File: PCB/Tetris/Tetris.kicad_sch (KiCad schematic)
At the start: 41 parts, among them J2 PWM, J3 Analog, J4 PWM, J5 Analog, J6 Communication, J7 Digital, M1 RGBMatrix, M2 RGBMatrix, SW1 SW_Push, SW2 SW_Push, SW3 SW_Push, SW4 SW_Push, SW5 SW_Push, SW6 SW_Push, SW7 SW_Push

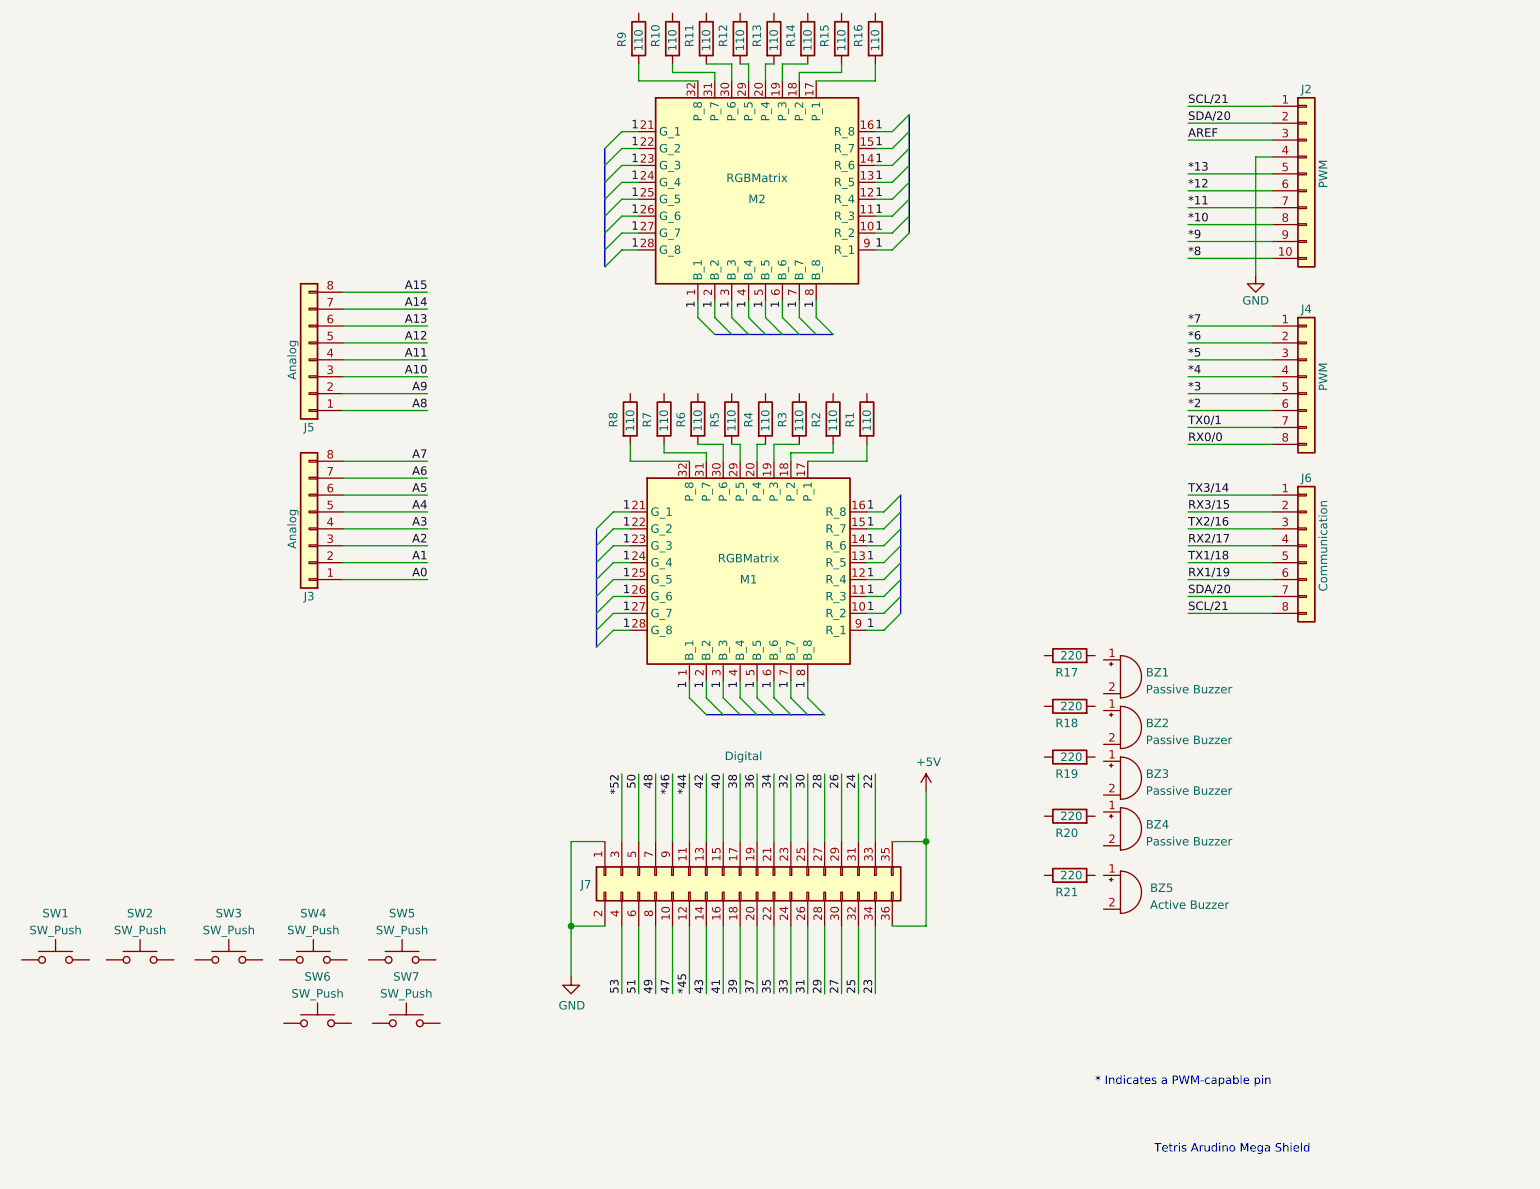
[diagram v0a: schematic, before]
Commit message: sync
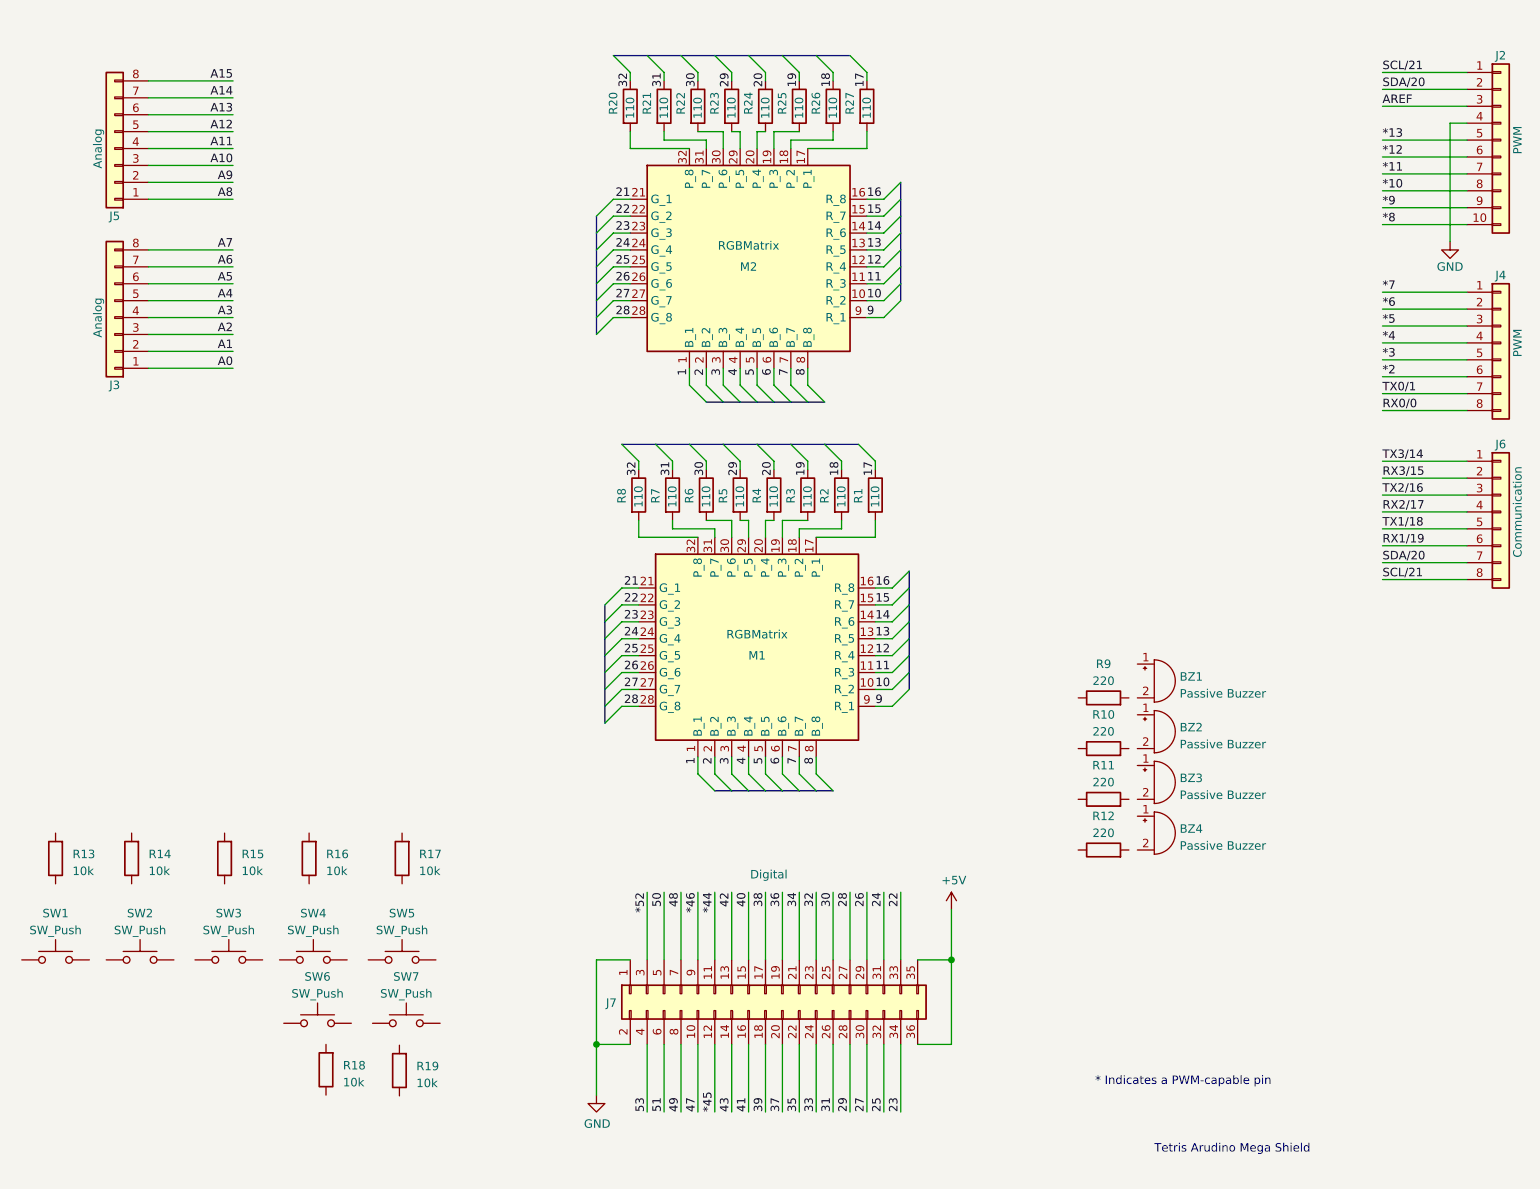
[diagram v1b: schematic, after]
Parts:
- removed BZ5: Active Buzzer, Buzzer_Beeper:MagneticBuzzer_PUI_AT-0927-TT-6-R, symbol Device:Buzzer
- added R22, R23, R24, R25, R26, R27: 110, Resistor_THT:R_Axial_DIN0207_L6.3mm_D2.5mm_P10.16mm_Horizontal, symbol Device:R
- BZ1, BZ2, BZ3, BZ4: footprint Buzzer_Beeper:MagneticBuzzer_PUI_AT-0927-TT-6-R -> Buzzer_Beeper:Buzzer_TDK_PS1240P02BT_D12.2mm_H6.5mm
- J2: footprint Connector_PinSocket_2.54mm:PinSocket_1x10_P2.54mm_Vertical -> Connector_PinHeader_2.54mm:PinHeader_1x10_P2.54mm_Vertical
- J4, J6: footprint Connector_PinSocket_2.54mm:PinSocket_1x08_P2.54mm_Vertical -> Connector_PinHeader_2.54mm:PinHeader_1x08_P2.54mm_Vertical
- R1, R2, R3, R4, R5, R6, R7, R8: footprint (none) -> Resistor_THT:R_Axial_DIN0207_L6.3mm_D2.5mm_P10.16mm_Horizontal
- R10, R11, R12, R9: value 110 -> 220; footprint (none) -> Resistor_THT:R_Axial_DIN0207_L6.3mm_D2.5mm_P10.16mm_Horizontal
- R13, R14, R15, R16: value 110 -> 10k; footprint (none) -> Resistor_THT:R_Axial_DIN0207_L6.3mm_D2.5mm_P10.16mm_Horizontal
- R17, R18, R19: value 220 -> 10k; footprint (none) -> Resistor_THT:R_Axial_DIN0207_L6.3mm_D2.5mm_P10.16mm_Horizontal
- R20, R21: value 220 -> 110; footprint (none) -> Resistor_THT:R_Axial_DIN0207_L6.3mm_D2.5mm_P10.16mm_Horizontal
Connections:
- net 1: no longer M1.10 (R_2), M1.11 (R_3), M1.12 (R_4), M1.13 (R_5), M1.14 (R_6), M1.15 (R_7), M1.16 (R_8), M1.2 (B_2), M1.21 (G_1), M1.22 (G_2), M1.23 (G_3), M1.24 (G_4), M1.25 (G_5), M1.26 (G_6), M1.27 (G_7), M1.28 (G_8), M1.3 (B_3), M1.4 (B_4), M1.5 (B_5), M1.6 (B_6), M1.7 (B_7), M1.8 (B_8), M1.9 (R_1), M2.10 (R_2), M2.11 (R_3), M2.12 (R_4), M2.13 (R_5), M2.14 (R_6), M2.15 (R_7), M2.16 (R_8), M2.2 (B_2), M2.21 (G_1), M2.22 (G_2), M2.23 (G_3), M2.24 (G_4), M2.25 (G_5), M2.26 (G_6), M2.27 (G_7), M2.28 (G_8), M2.3 (B_3), M2.4 (B_4), M2.5 (B_5), M2.6 (B_6), M2.7 (B_7), M2.8 (B_8), M2.9 (R_1)
- net 22: now also M1.22 (G_2), M2.22 (G_2)
- net 23: now also M1.23 (G_3), M2.23 (G_3)
- net 24: now also M1.24 (G_4), M2.24 (G_4)
- net 25: now also M1.25 (G_5), M2.25 (G_5)
- net 26: now also M1.26 (G_6), M2.26 (G_6)
- net 27: now also M1.27 (G_7), M2.27 (G_7)
- net 28: now also M1.28 (G_8), M2.28 (G_8)
- net 29: now also R5.1, R23.1
- net 30: now also R6.1, R22.1
- net 31: now also R21.1, R7.1
- net 32: now also R20.1, R8.1
- net at R16.2: no longer M2.17 (P_1)
- net at R10.2: no longer M2.31 (P_7)
- net at M2.29 (P_5): now also R23.2; no longer R12.2
- net at M2.18 (P_2): now also R26.2; no longer R15.2
- net at M2.19 (P_3): now also R25.2; no longer R14.2
- net at M2.20 (P_4): now also R24.2; no longer R13.2
- net at M2.30 (P_6): now also R22.2; no longer R11.2
- net at M2.32 (P_8): now also R20.2; no longer R9.2
- net 20: now reaches R4.1
- net 20: now also R24.1
- net 19: now reaches R3.1
- net 19: now also R25.1
- net 18: now reaches R2.1
- net 18: now also R26.1
- net 17: now reaches R1.1
- net 17: now also R27.1
- net at R21.2: now also M2.31 (P_7)
- new net: M2.17 (P_1), R27.2
- new net 10: M1.10 (R_2), M2.10 (R_2)
- new net 11: M1.11 (R_3), M2.11 (R_3)
- new net 12: M1.12 (R_4), M2.12 (R_4)
- new net 13: M1.13 (R_5), M2.13 (R_5)
- new net 14: M1.14 (R_6), M2.14 (R_6)
- new net 15: M1.15 (R_7), M2.15 (R_7)
- new net 16: M1.16 (R_8), M2.16 (R_8)
- new net 2: M1.2 (B_2), M2.2 (B_2)
- new net 21: M1.21 (G_1), M2.21 (G_1)
- new net 3: M1.3 (B_3), M2.3 (B_3)
- new net 4: M1.4 (B_4), M2.4 (B_4)
- new net 5: M1.5 (B_5), M2.5 (B_5)
- new net 6: M1.6 (B_6), M2.6 (B_6)
- new net 7: M1.7 (B_7), M2.7 (B_7)
- new net 8: M1.8 (B_8), M2.8 (B_8)
- new net 9: M1.9 (R_1), M2.9 (R_1)
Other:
- moved on the sheet: BZ1, BZ2, BZ3, BZ4, J2, J3, J4, J5, J6, J7, M1, R1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

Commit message: Making diabolical progress
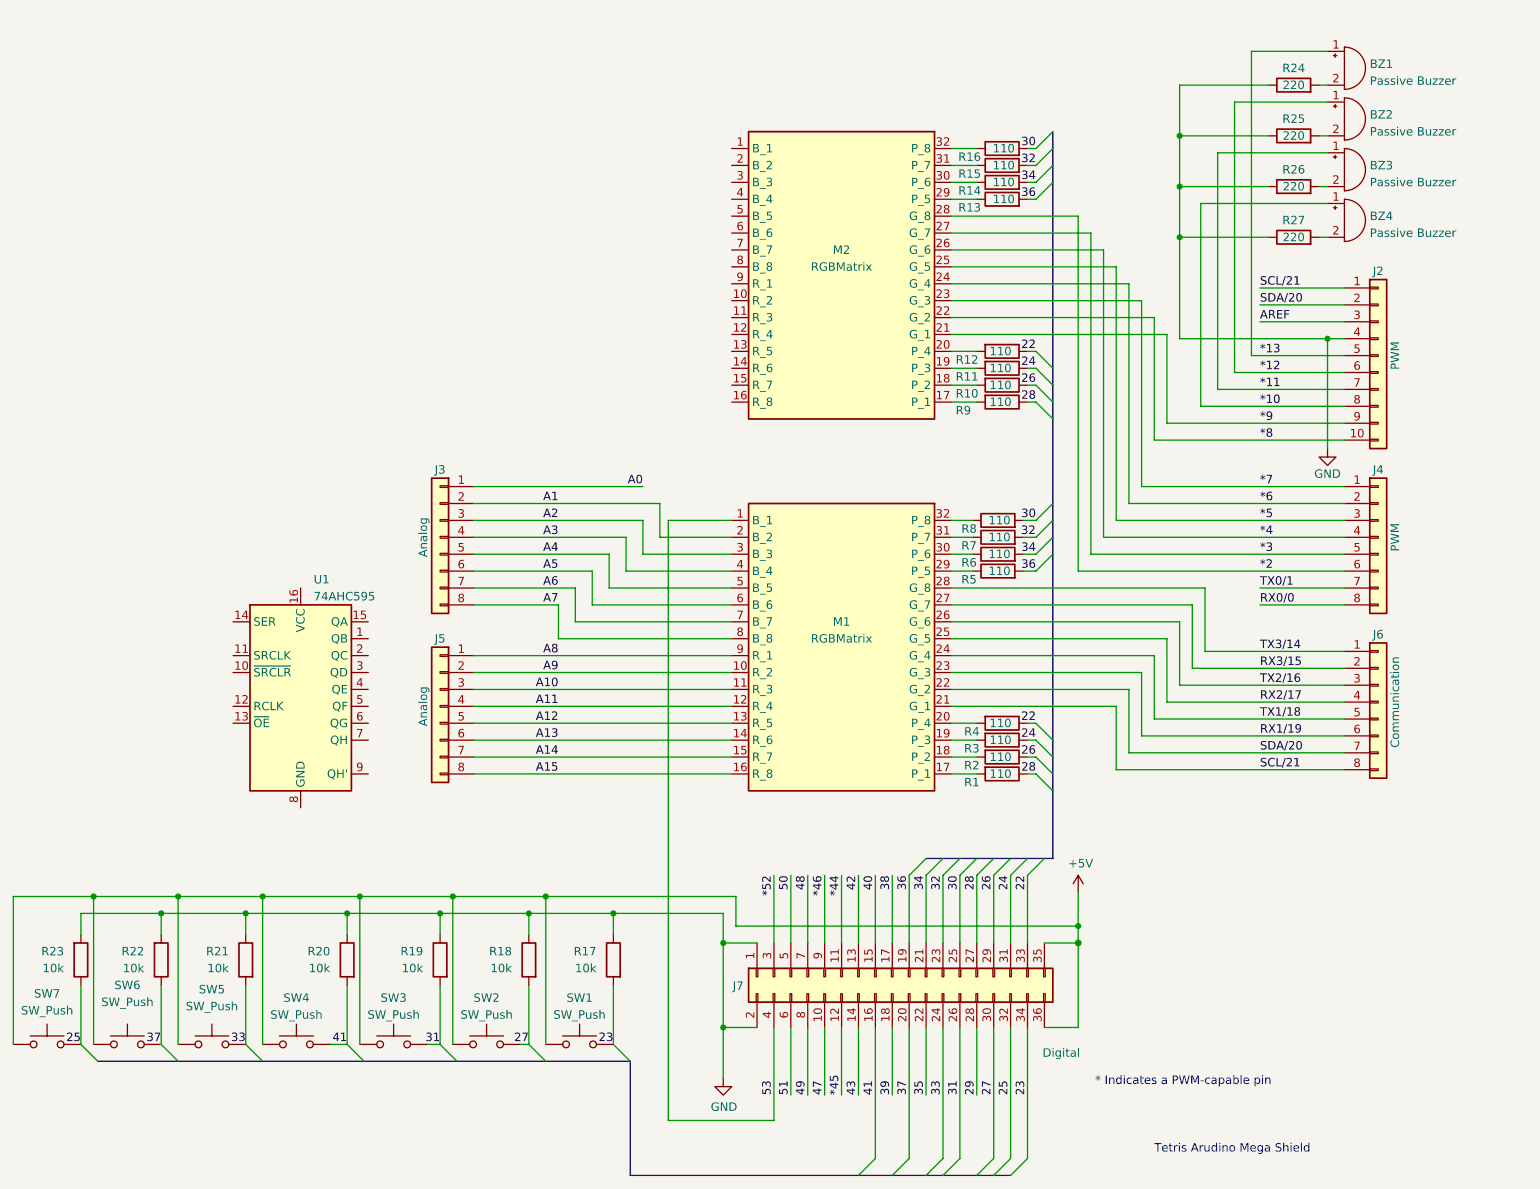
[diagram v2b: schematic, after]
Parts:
- removed R20, R21, R22, R23, R24, R25, R26, R27: 110, Resistor_THT:R_Axial_DIN0207_L6.3mm_D2.5mm_P10.16mm_Horizontal, symbol Device:R
- added R10, R11, R12, R13, R14, R15, R16, R9: 110, Resistor_THT:R_Axial_DIN0207_L6.3mm_D2.5mm_P10.16mm_Horizontal, symbol Device:R
- added U1: 74AHC595, Package_DIP:DIP-16_W7.62mm_Socket_LongPads, symbol 74xx:74AHC595
- J3, J5: footprint Connector_PinSocket_2.54mm:PinSocket_1x08_P2.54mm_Vertical -> Connector_PinHeader_2.54mm:PinHeader_1x08_P2.54mm_Vertical
- J7: footprint Connector_PinSocket_2.54mm:PinSocket_2x18_P2.54mm_Vertical -> Connector_PinHeader_2.54mm:PinHeader_2x18_P2.54mm_Vertical
- renumbered R13 to R17, R14 to R18, R15 to R19, R16 to R20, R17 to R21, R18 to R22, R19 to R23, R9 to R24, R10 to R25, R11 to R26, R12 to R27, R8 to R5, R7 to R6, R6 to R7, R5 to R8
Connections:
- net 17 is gone; now on net 28: R1.1
- net 18 is gone; now on net 26: R2.1
- net 19 is gone; now on net 24: R3.1
- net 20 is gone; now on net 22: R4.1
- net *10: now also BZ4.1 (-)
- net *11: now also BZ3.1 (-)
- net *12: now also BZ2.1 (-)
- net *13: now also BZ1.1 (-)
- net *2: now also M2.28 (G_8)
- net *3: now also M2.27 (G_7)
- net *4: now also M2.26 (G_6)
- net *5: now also M2.25 (G_5)
- net *6: now also M2.24 (G_4)
- net *7: now also M2.23 (G_3)
- net *8: now also M2.22 (G_2)
- net *9: now also M2.21 (G_1)
- net +5V: now also SW1.2, SW2.2, SW3.2, SW4.2, SW5.2, SW6.2, SW7.2
- net 22: now also R12.1; no longer M1.22 (G_2), M2.22 (G_2)
- net 23: now also R17.2, SW1.1; no longer M1.23 (G_3), M2.23 (G_3)
- net 24: now also R11.1; no longer M1.24 (G_4), M2.24 (G_4)
- net 25: now also R23.1, SW7.1; no longer M1.25 (G_5), M2.25 (G_5)
- net 26: now also R10.1; no longer M1.26 (G_6), M2.26 (G_6)
- net 27: now also R18.2, SW2.1; no longer M1.27 (G_7), M2.27 (G_7)
- net 28: now also R9.1; no longer M1.28 (G_8), M2.28 (G_8)
- net 29: no longer R8.1
- net 30: now also R8.2, R16.2; no longer R7.1
- net 31: now also R19.2, SW3.1; no longer R6.1
- net 32: now also R7.2, R15.2; no longer R5.1
- net 33: now also R21.2, SW5.1
- net 34: now also R6.2, R14.2
- net 36: now also R5.2, R13.2
- net 37: now also R22.1, SW6.1
- net 41: now also R20.2, SW4.1
- net 53: now also M1.1 (B_1)
- net A1: now also M1.2 (B_2)
- net A10: now also M1.11 (R_3)
- net A11: now also M1.12 (R_4)
- net A12: now also M1.13 (R_5)
- net A13: now also M1.14 (R_6)
- net A14: now also M1.15 (R_7)
- net A15: now also M1.16 (R_8)
- net A2: now also M1.3 (B_3)
- net A3: now also M1.4 (B_4)
- net A4: now also M1.5 (B_5)
- net A5: now also M1.6 (B_6)
- net A6: now also M1.7 (B_7)
- net A7: now also M1.8 (B_8)
- net A8: now also M1.9 (R_1)
- net A9: now also M1.10 (R_2)
- net GND: now also R17.1, R18.1, R19.1, R20.1, R21.1, R22.2, R23.2, R24.1, R25.1, R26.1, R27.1
- net RX1/19: now also M1.23 (G_3)
- net RX2/17: now also M1.25 (G_5)
- net RX3/15: now also M1.27 (G_7)
- net SCL/21: now also M1.21 (G_1)
- net SDA/20: now also M1.22 (G_2)
- net TX1/18: now also M1.24 (G_4)
- net TX2/16: now also M1.26 (G_6)
- net TX3/14: now also M1.28 (G_8)
- net at BZ1.2 (+): now also R24.2
- net at M2.20 (P_4): now also R12.2
- net at R25.2: now also BZ2.2 (+)
- net at BZ3.2 (+): now also R26.2
- net at M2.17 (P_1): now also R9.2
- net at M2.18 (P_2): now also R10.2
- net at M2.19 (P_3): now also R11.2
- net at M2.29 (P_5): now also R13.1
- net at M2.30 (P_6): now also R14.1
- net at M2.31 (P_7): now also R15.1
- net at M2.32 (P_8): now also R16.1
- net at M1.32 (P_8): now also R8.1; no longer R5.2
- net at M1.31 (P_7): now also R7.1; no longer R6.2
- net at M1.30 (P_6): now also R6.1; no longer R7.2
- net at BZ4.2 (+): now also R27.2
- net at M1.29 (P_5): now also R5.1; no longer R8.2
- net 1: no longer names the net of M2.1 (B_1)
- net 1: no longer M1.1 (B_1)
- net 10: no longer names the net of M2.10 (R_2)
- net 10: no longer M1.10 (R_2)
- net 11: no longer names the net of M2.11 (R_3)
- net 11: no longer M1.11 (R_3)
- net 12: no longer names the net of M2.12 (R_4)
- net 12: no longer M1.12 (R_4)
- net 13: no longer names the net of M2.13 (R_5)
- net 13: no longer M1.13 (R_5)
- net 14: no longer names the net of M2.14 (R_6)
- net 14: no longer M1.14 (R_6)
- net 15: no longer names the net of M2.15 (R_7)
- net 15: no longer M1.15 (R_7)
- net 16: no longer names the net of M2.16 (R_8)
- net 16: no longer M1.16 (R_8)
- net 2: no longer names the net of M2.2 (B_2)
- net 2: no longer M1.2 (B_2)
- removed net 21: M1.21 (G_1), M2.21 (G_1)
- net 3: no longer names the net of M2.3 (B_3)
- net 3: no longer M1.3 (B_3)
- net 4: no longer names the net of M2.4 (B_4)
- net 4: no longer M1.4 (B_4)
- net 5: no longer names the net of M2.5 (B_5)
- net 5: no longer M1.5 (B_5)
- net 6: no longer names the net of M2.6 (B_6)
- net 6: no longer M1.6 (B_6)
- net 7: no longer names the net of M2.7 (B_7)
- net 7: no longer M1.7 (B_7)
- net 8: no longer names the net of M2.8 (B_8)
- net 8: no longer M1.8 (B_8)
- net 9: no longer names the net of M2.9 (R_1)
- net 9: no longer M1.9 (R_1)
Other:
- moved on the sheet: BZ1, BZ2, BZ3, BZ4, J2, J3, J4, J5, J6, J7, M1, R1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
